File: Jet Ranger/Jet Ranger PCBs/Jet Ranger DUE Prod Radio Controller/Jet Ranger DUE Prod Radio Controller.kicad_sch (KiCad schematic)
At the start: 60 parts, among them J1 ANNODES, J12 AUTOPILOT, J15 Conn_01x02, J2 Conn_01x03_Pin, J3 RS232 OUT, J4 5V IN, J40 Conn_01x08, J41 Conn_01x08, J42 Conn_01x08, J43 Conn_01x08, J44 Conn_01x08, J45 Conn_01x10, J5 NAV_COMM, J50 Conn_01x02, J51 Conn_01x02, J6 CATHODES, J7 STEPPER IN 12-20VDC, J8 DOUT, J9 Keypad, Q5 Q_NMOS_GSD, U1 USR-ES1, U2 MAX7219, U3 TCA9548APWR, U4 ULN2803A, U5 MAX232

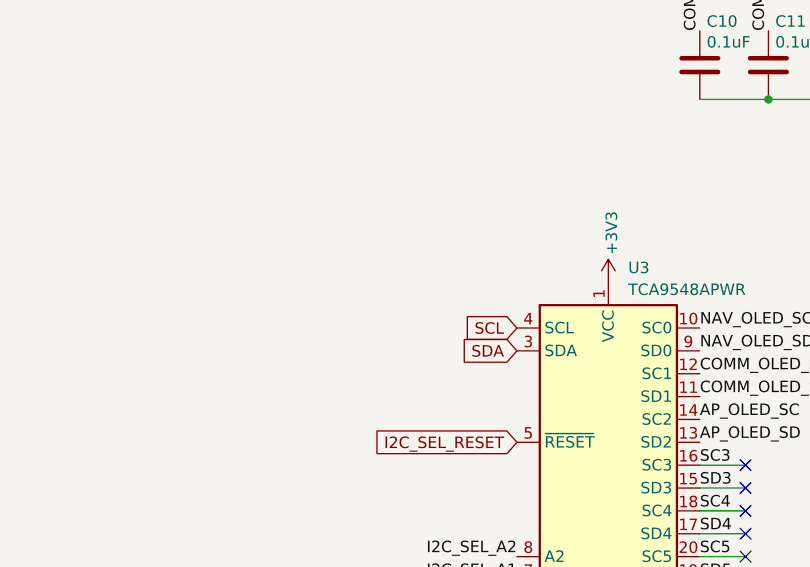
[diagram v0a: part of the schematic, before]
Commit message: due controller
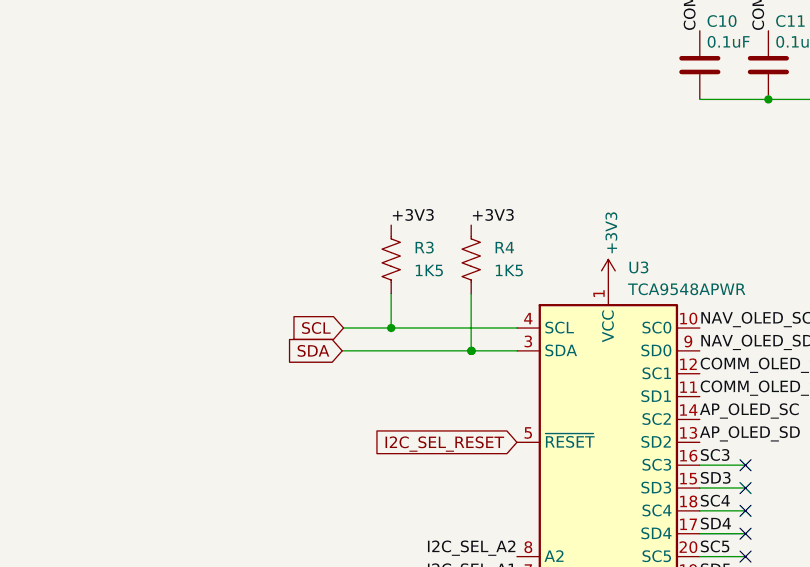
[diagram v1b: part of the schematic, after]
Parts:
- added R3, R4: 1K5, Resistor_THT:R_Axial_DIN0207_L6.3mm_D2.5mm_P2.54mm_Vertical, symbol Device:R_US
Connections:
- net +3V3: now also R3.1, R4.1
- net SCL: now also R3.2
- net SDA: now also R4.2
